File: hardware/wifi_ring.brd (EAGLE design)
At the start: 65 x 30 mm, 60 parts, among them IC1 ESP-12E/F, IC2 FT230XS, IC3 LD117ADT33TR, Q1 BC847BS, Q2 BC847BS, Q3 BC847BS, Q4 IRLML5203, X1 MINI-USB-UX60-MB-5ST

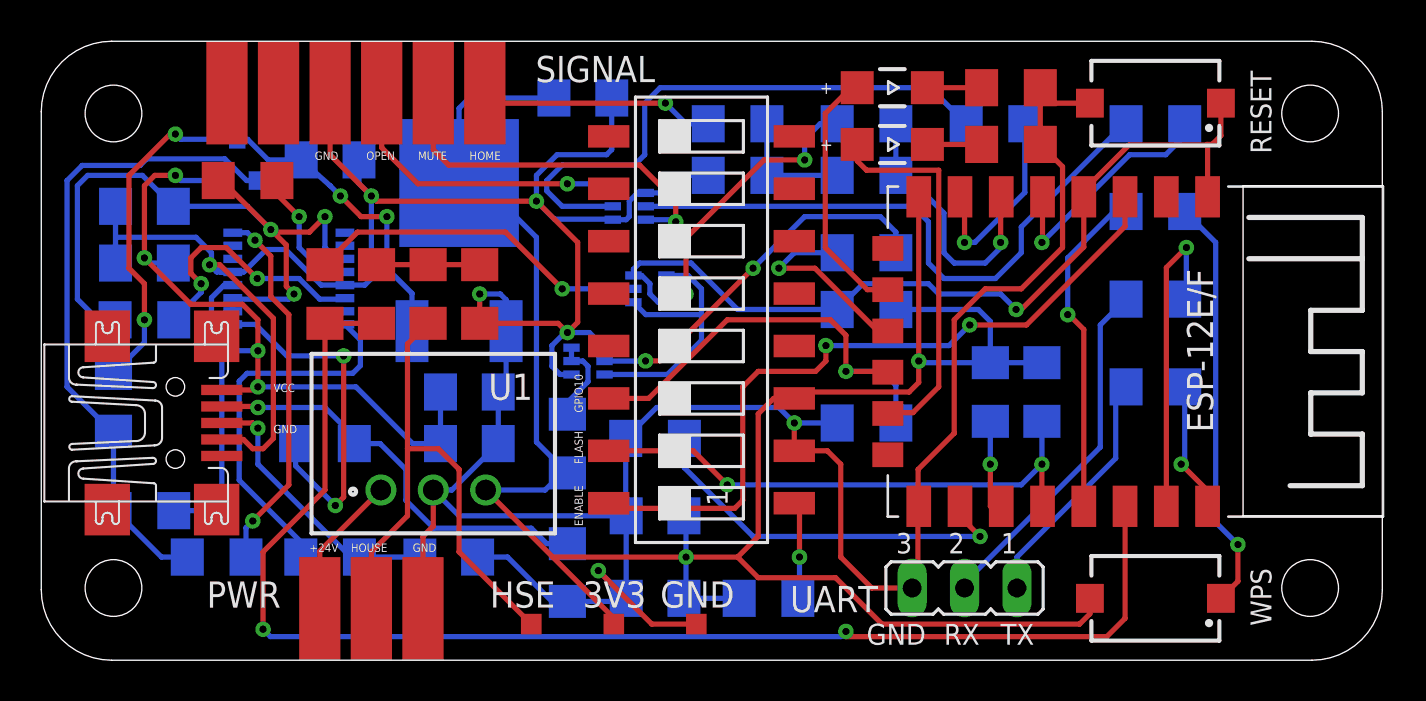
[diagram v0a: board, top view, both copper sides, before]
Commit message: Adding latest layout changes for eurocircuits order
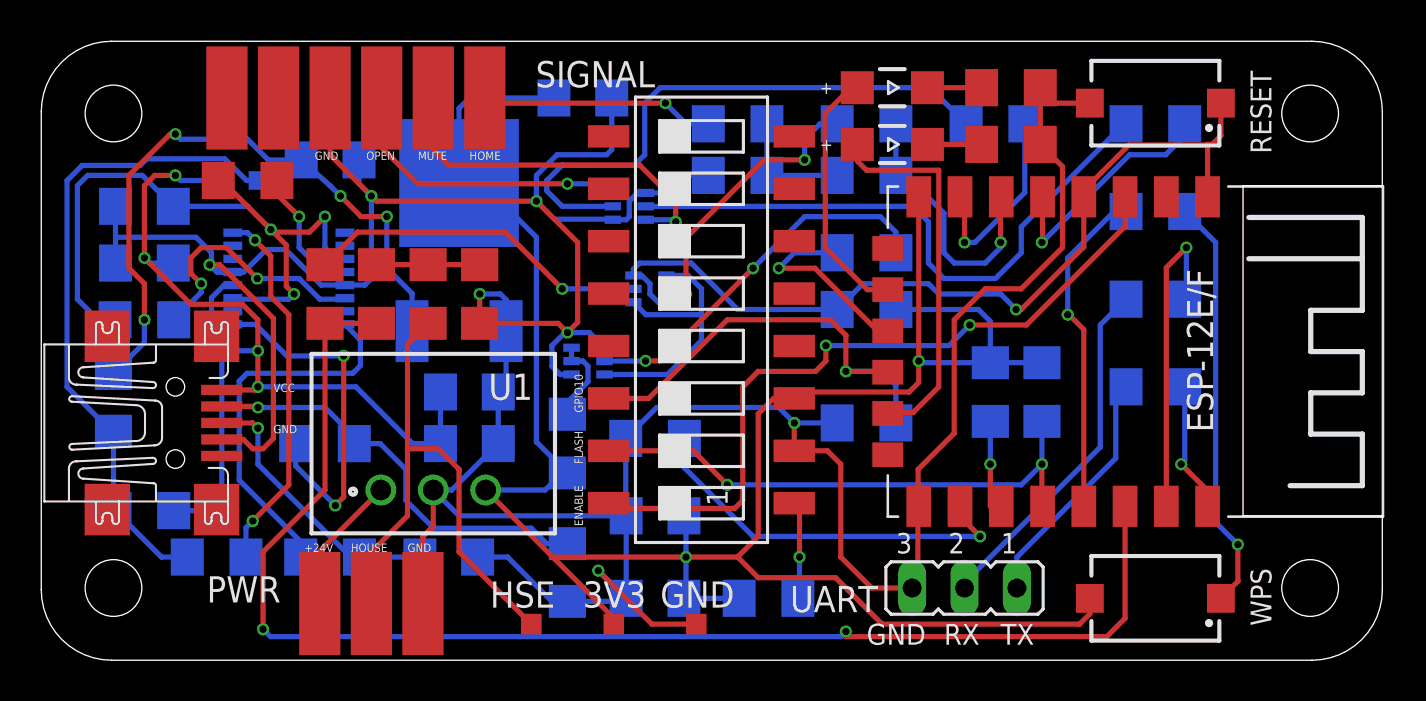
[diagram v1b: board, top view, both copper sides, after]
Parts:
- moved PWR 0.25 mm to (16.0, 2.75)
- moved SIGNAL 0.25 mm to (15.5, 27.2)
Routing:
- net GND: track 195.3 -> 194.7 mm
